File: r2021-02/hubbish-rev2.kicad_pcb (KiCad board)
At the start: 4 copper layers, 103.6 x 71.8 mm, 100 parts, among them J1 Conn_01x06, J10 USB_A_DUAL, J4 USB_A (female down), J5 Conn_01x03_Male, J6 USB_A_DUAL, J7 USB_A_DUAL, J8 USB_A male UP, J9 USB_B_Micro (up), U1 2k i2c eeprom, U10 NUP4202, U11 NUP4202, U12 NUP4202, U13 NUP4202, U14 NUP4202, U15 NUP4202, U16 NUP4202, U17 NUP4202, U18 SY8366H, U2 SE5120ST33, U3 USB2517, U4 APL3511C, U5 APL3511C, U6 APL3511C, U7 APL3511C, U8 APL3511C, U9 APL3511C, Y1 24MHz

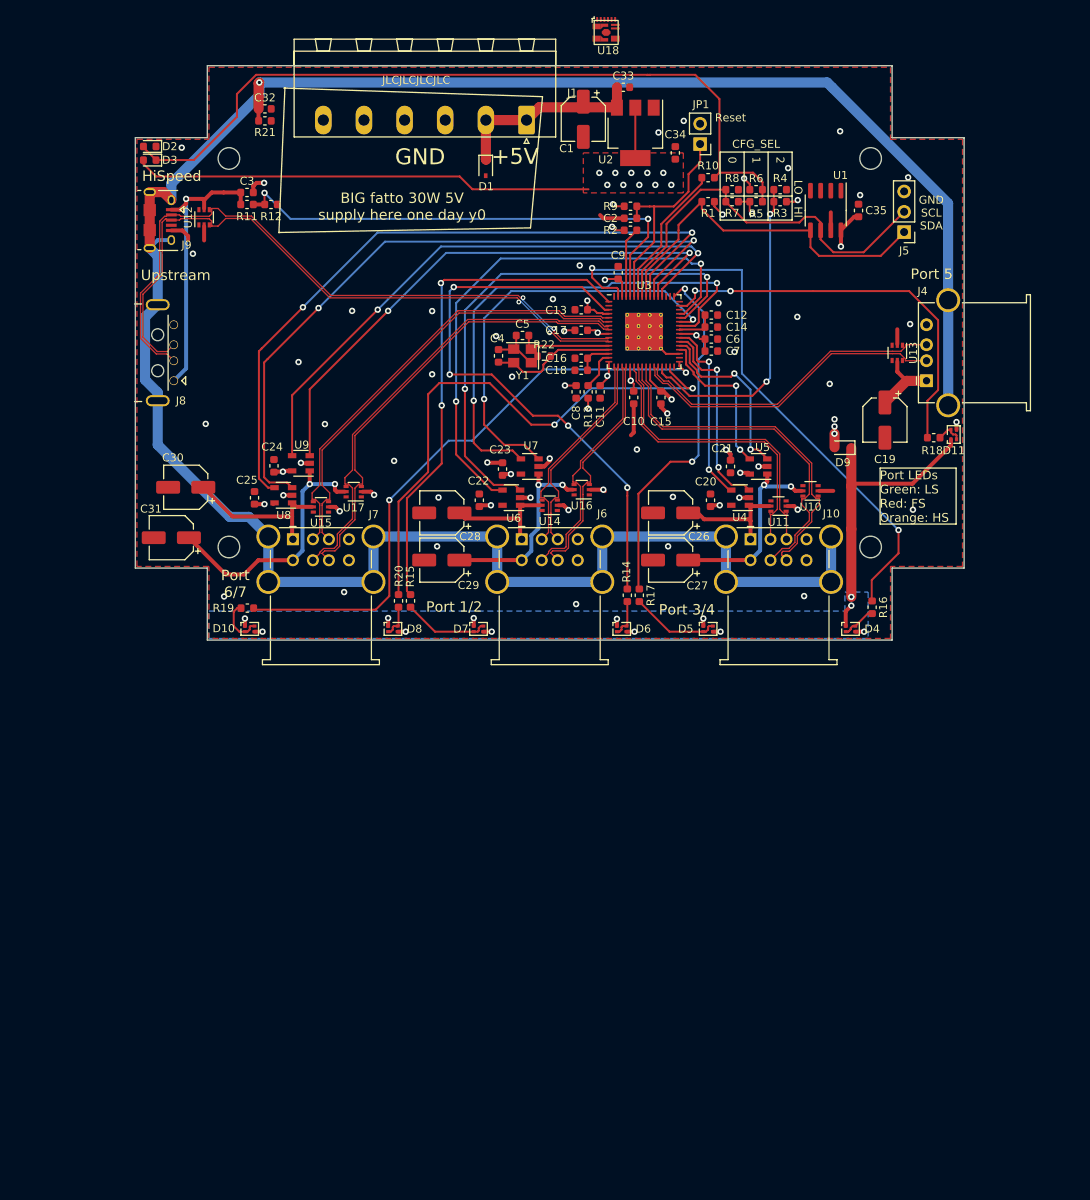
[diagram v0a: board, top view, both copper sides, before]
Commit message: start rev2
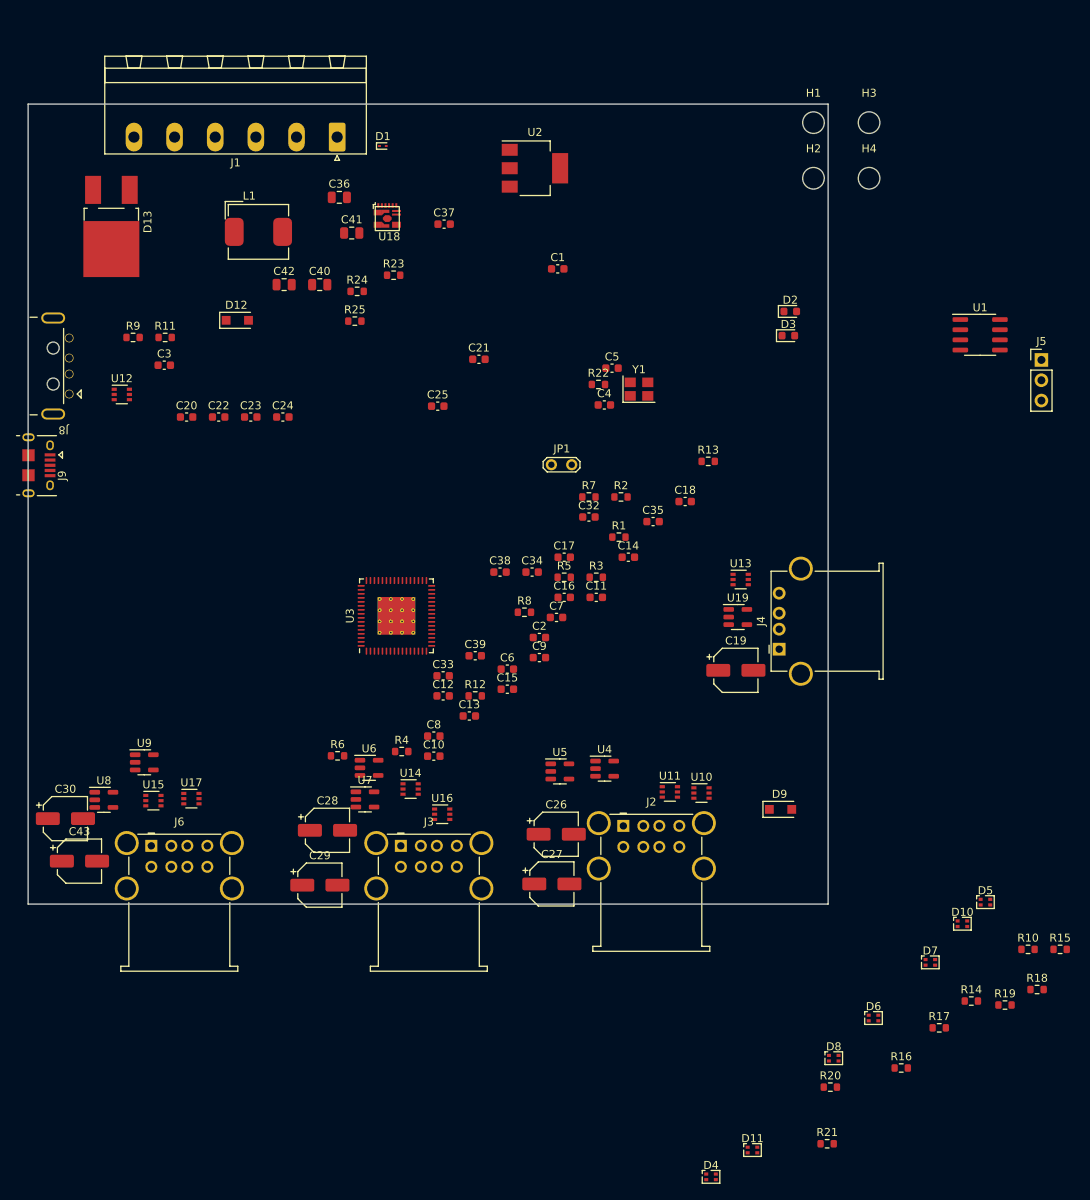
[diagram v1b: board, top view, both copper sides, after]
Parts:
- removed C31: 100uF, Capacitor_SMD:CP_Elec_5x5.4
- removed J10, J7: USB_A_DUAL, Connector_USB:USB_A_Wuerth_61400826021_Horizontal_Stacked
- added C36: 10uF/50V, Capacitor_SMD:C_0805_2012Metric, F.Cu at (118.9, 61.7)
- added C37: 2.2uF, Capacitor_SMD:C_0603_1608Metric, F.Cu at (132.0, 65.0)
- added C38: 100nF, Capacitor_SMD:C_0603_1608Metric, F.Cu at (139.0, 108.5)
- added C39: Cff, Capacitor_SMD:C_0603_1608Metric, F.Cu at (135.9, 119.0)
- added C40: 22uF/6.3V, Capacitor_SMD:C_0805_2012Metric, F.Cu at (116.5, 72.6)
- added C41: 22uF/6.3V, Capacitor_SMD:C_0805_2012Metric, F.Cu at (120.5, 66.1)
- added C42: 22uF/6.3V, Capacitor_SMD:C_0805_2012Metric, F.Cu at (112.0, 72.6)
- added C43: 100uF, Capacitor_SMD:CP_Elec_5x5.4, F.Cu at (86.4, 144.6)
- added D12: SMF24A, Diode_SMD:D_SOD-123F, F.Cu at (106.2, 77.0)
- added D13: MBR1040, Package_TO_SOT_SMD:TO-252-2_TabPin1, F.Cu at (90.4, 65.3)
- added J2: USB_A_Stacked, Connector_USB:USB_A_Wuerth_61400826021_Horizontal_Stacked, F.Cu at (154.4, 140.2)
- added J3: USB_A_Stacked, Connector_USB:USB_A_Wuerth_61400826021_Horizontal_Stacked, F.Cu at (126.6, 142.7)
- added L1: 2.2uH, Inductor_SMD:L_CHILISIN_BMRx00060630, F.Cu at (108.8, 66.0)
- added R23: Rff, Resistor_SMD:R_0603_1608Metric, F.Cu at (125.7, 71.4)
- added R24: 100k/1%, Resistor_SMD:R_0603_1608Metric, F.Cu at (121.1, 73.4)
- added R25: 13k6/1%, Resistor_SMD:R_0603_1608Metric, F.Cu at (120.8, 77.1)
- added U19: APL3511C, Package_TO_SOT_SMD:SOT-23-5, F.Cu at (168.7, 114.1)
- C1: value 100uF -> 1uF; footprint Capacitor_SMD:CP_Elec_5x5.4 -> Capacitor_SMD:C_0603_1608Metric
- D1: value SD05-7 -> DF2S6.2FS,L3M; footprint Diode_SMD:D_SOD-323 -> Diode_SMD:D_SOD-923
- D9: value D_Small -> SM400x; footprint Diode_SMD:D_SOD-323 -> Diode_SMD:D_SOD-123F
- J6: value USB_A_DUAL -> USB_A_Stacked
- JP1: value Jumper_NO_Small -> Jumper_2_Open; footprint Connector_PinHeader_2.54mm:PinHeader_1x02_P2.54mm_Vertical -> TestPoint:TestPoint_2Pads_Pitch2.54mm_Drill0.8mm
- moved R21 145.9 mm to (179.9, 180.0), turned to 0 degrees
- moved R19 106.9 mm to (202.1, 162.6), turned to 0 degrees
- moved R10 104.4 mm to (205.0, 155.7), turned to 0 degrees
- moved D10 96.4 mm to (196.8, 152.5)
- moved D11 92.9 mm to (170.5, 180.7), turned to 0 degrees
- moved R15 92.1 mm to (209.0, 155.7), turned to 0 degrees
- moved R6 88.0 mm to (118.7, 131.5), turned to 0 degrees
- moved H2 86.4 mm to (178.2, 59.3)
- moved R4 84.7 mm to (126.7, 130.9)
- moved D3 82.8 mm to (175.0, 79.0), turned to 0 degrees
- moved D2 82.7 mm to (175.3, 75.9), turned to 0 degrees
- moved R20 81.3 mm to (180.3, 172.9), turned to 0 degrees
- moved C33 76.9 mm to (131.9, 121.5)
- moved D8 76.9 mm to (180.7, 169.3)
- moved H1 73.2 mm to (178.2, 52.3)
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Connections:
- C19 pad 1: +5V -> /downstream-port-power/VBUS_DS
- J1 pad 6: (no net) -> Net-(D13-Pad2)
- J4 pad 1: +5V -> /downstream-port-power/VBUS_DS
- J5 pad 2: /upstream-config-leds/CFG_SEL0 -> /upstream-config-leds/EE_SCL
- J6 pad 1: /downstream-port-power/VBUS3 -> /downstream-port-power/VBUS5
- J6 pad 2: /downstream-port-power/U3- -> /downstream-port-power/U5-
- J6 pad 3: /downstream-port-power/U3+ -> /downstream-port-power/U5+
- J6 pad 5: /downstream-port-power/VBUS4 -> /downstream-port-power/VBUS6
- J6 pad 6: /downstream-port-power/U4- -> /downstream-port-power/U6-
- J6 pad 7: /downstream-port-power/U4+ -> /downstream-port-power/U6+
- R7 pad 2: /upstream-config-leds/CFG_SEL0 -> /upstream-config-leds/CFG_SEL0-EE_SCL
- R8 pad 1: /upstream-config-leds/CFG_SEL0 -> /upstream-config-leds/CFG_SEL0-EE_SCL
- U1 pad 6: /upstream-config-leds/CFG_SEL0 -> /upstream-config-leds/EE_SCL
- U10 pad 3: unconnected-(U10-Pad3) -> (no net)
- U10 pad 4: unconnected-(U10-Pad4) -> (no net)
- U11 pad 3: unconnected-(U11-Pad3) -> (no net)
- U11 pad 4: unconnected-(U11-Pad4) -> (no net)
- U12 pad 1: unconnected-(U12-Pad1) -> (no net)
- U12 pad 6: unconnected-(U12-Pad6) -> (no net)
- U13 pad 3: unconnected-(U13-Pad3) -> (no net)
- U13 pad 4: unconnected-(U13-Pad4) -> (no net)
- U14 pad 1: unconnected-(U14-Pad1) -> (no net)
- U14 pad 6: unconnected-(U14-Pad6) -> (no net)
- U15 pad 1: unconnected-(U15-Pad1) -> (no net)
- U15 pad 6: unconnected-(U15-Pad6) -> (no net)
- U16 pad 1: unconnected-(U16-Pad1) -> (no net)
- U16 pad 6: unconnected-(U16-Pad6) -> (no net)
- U17 pad 1: unconnected-(U17-Pad1) -> (no net)
- U17 pad 6: unconnected-(U17-Pad6) -> (no net)
- U18 pad 1: unconnected-(U18-Pad1) -> GND
- U18 pad 10: unconnected-(U18-Pad10) -> (no net)
- U18 pad 11: unconnected-(U18-Pad11) -> (no net)
- U18 pad 12: unconnected-(U18-Pad12) -> +VDC
- U18 pad 2: unconnected-(U18-Pad2) -> Net-(C38-Pad2)
- U18 pad 5: (no net) -> +VDC
- U18 pad 6: (no net) -> +VDC
- U18 pad 7: unconnected-(U18-Pad7) -> Net-(C38-Pad1)
- U18 pad 8: unconnected-(U18-Pad8) -> Net-(C37-Pad1)
- U18 pad 9: unconnected-(U18-Pad9) -> Net-(R23-Pad1)
- U3 pad 14: unconnected-(U3-Pad14) -> (no net)
- U3 pad 16: unconnected-(U3-Pad16) -> (no net)
- U3 pad 18: unconnected-(U3-Pad18) -> (no net)
- U3 pad 30: unconnected-(U3-Pad30) -> /downstream-port-power/EN_DS
- U3 pad 32: unconnected-(U3-Pad32) -> (no net)
- U3 pad 34: unconnected-(U3-Pad34) -> (no net)
- U3 pad 35: unconnected-(U3-Pad35) -> /downstream-port-power/OC_DS
- U3 pad 41: /upstream-config-leds/CFG_SEL0 -> /upstream-config-leds/CFG_SEL0-EE_SCL
- U3 pad 48: unconnected-(U3-Pad48) -> (no net)
- U3 pad 50: unconnected-(U3-Pad50) -> (no net)
- U3 pad 60: Net-(C4-Pad1) -> (no net)
- U3 pad 61: Net-(C5-Pad2) -> (no net)
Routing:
- net GNDPWR: track 306.4 -> 0.00 mm, vias 1 -> 0
- net +3V3: track 109.4 -> 0.00 mm, vias 27 -> 0
- net /upstream-config-leds/CFG_SEL1: track 98.5 -> 0.00 mm
- net /downstream-port-power/EN5: track 89.0 -> 0.00 mm, vias 2 -> 0
- net /downstream-port-power/OC5: track 87.8 -> 0.00 mm, vias 2 -> 0
- net /upstream-config-leds/UP-: track 85.4 -> 0.00 mm, vias 2 -> 0
- net /upstream-config-leds/UP+: track 84.4 -> 0.00 mm, vias 2 -> 0
- net GND: track 77.4 -> 0.00 mm, vias 59 -> 0
- net /upstream-config-leds/LED_A3: track 75.7 -> 0.00 mm, vias 2 -> 0
- net /upstream-config-leds/LED_A6: track 75.4 -> 0.00 mm, vias 2 -> 0
- net /downstream-port-power/EN6: track 73.6 -> 0.00 mm, vias 2 -> 0
- net /upstream-config-leds/LED_A1: track 72.6 -> 0.00 mm, vias 4 -> 0
- net /downstream-port-power/OC6: track 69.9 -> 0.00 mm, vias 2 -> 0
- net /upstream-config-leds/LED_A7: track 68.5 -> 0.00 mm, vias 2 -> 0
- net /downstream-port-power/EN3: track 67.5 -> 0.00 mm, vias 2 -> 0
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- removed copper zone on F.Cu, net +3V3
- removed copper zone on In2.Cu, net +3V3
- removed copper zone on In2.Cu, net +5V
- removed copper zone on B.Cu, net /upstream-config-leds/LED_DRIVE
- removed copper zone on F.Cu, net GND
- removed copper zone on In1.Cu, net GND
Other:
- board size 103.6 x 71.8 mm -> 100 x 100 mm
- copper layers 4 -> 2
- board text removed: "+5V"
- board text removed: "0"
- board text removed: "1"
- board text removed: "2"
- board text removed: "BIG fatto 30W 5V supply here one day y0"
- board text removed: "CFG_SEL"
- board text removed: "GND"
- board text removed: "GND SCL SDA"
- board text removed: "HI"
- board text removed: "HiSpeed"
- board text removed: "JLCJLCJLCJLC"
- board text removed: "JLCPCB 2313 stackup!"
- board text removed: "LO"
- board text removed: "Port 1/2"
- board text removed: "Port 3/4"
- board text removed: "Port 5"
- board text removed: "Port 6/7"
- board text removed: "Port LEDs Green: LS Red: FS Orange: HS"
- board text removed: "Reset"
- board text removed: "Upstream"
- board text removed: "github.com/karlp/hubbish rev 2020-03"
